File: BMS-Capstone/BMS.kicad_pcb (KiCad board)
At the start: 2 copper layers, 92.7 x 127 mm, 146 parts, among them IC1 BQ7694204PFBR, IC1 MP2643, IC2 MP2643, IC3 MP2643, IC4 MP2643, IC5 MP2643, IC6 MP2643, J1 Conn_01x02_Socket, J2 Conn_01x02_Socket, J3 Conn_01x13_Socket, K1 J107F1CS203VDC.80, Q1 FODM121, Q10 FODM121, Q11 FODM121, Q12 FODM121, Q2 FODM121, Q3 FODM121, Q4 FODM121, Q5 FODM121, Q6 FODM121, Q7 FODM121, Q8 FODM121, Q9 FODM121, U1 Teensy4.0

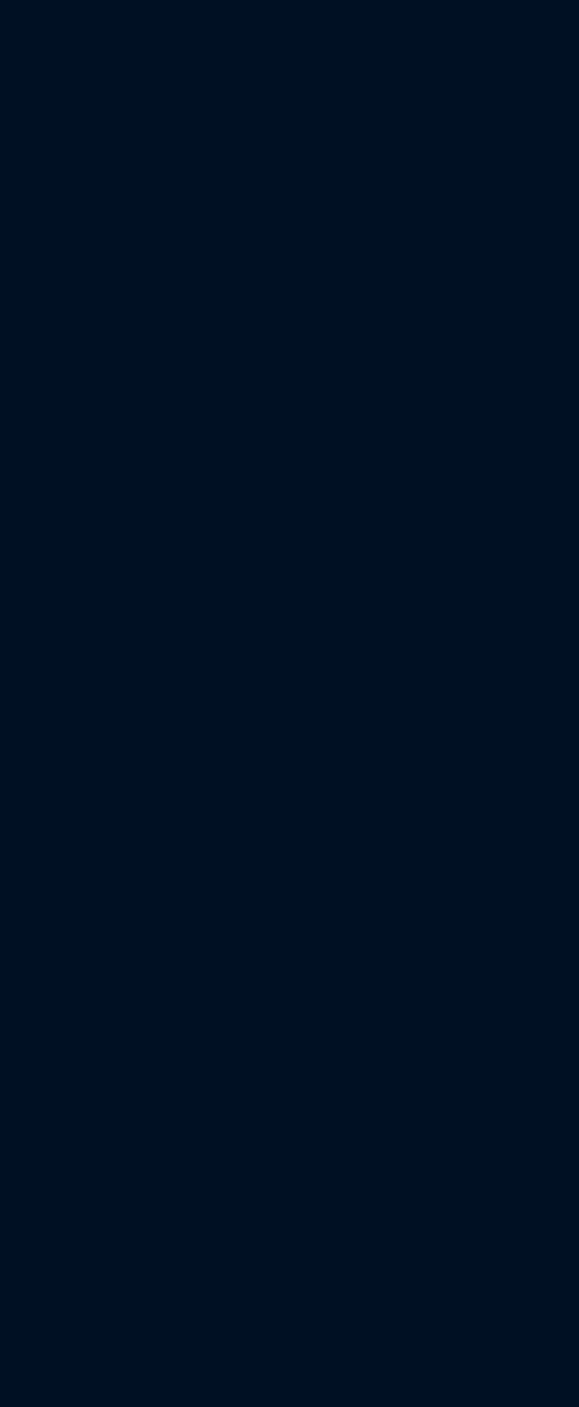
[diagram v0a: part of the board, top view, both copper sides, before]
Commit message: relinked footprints
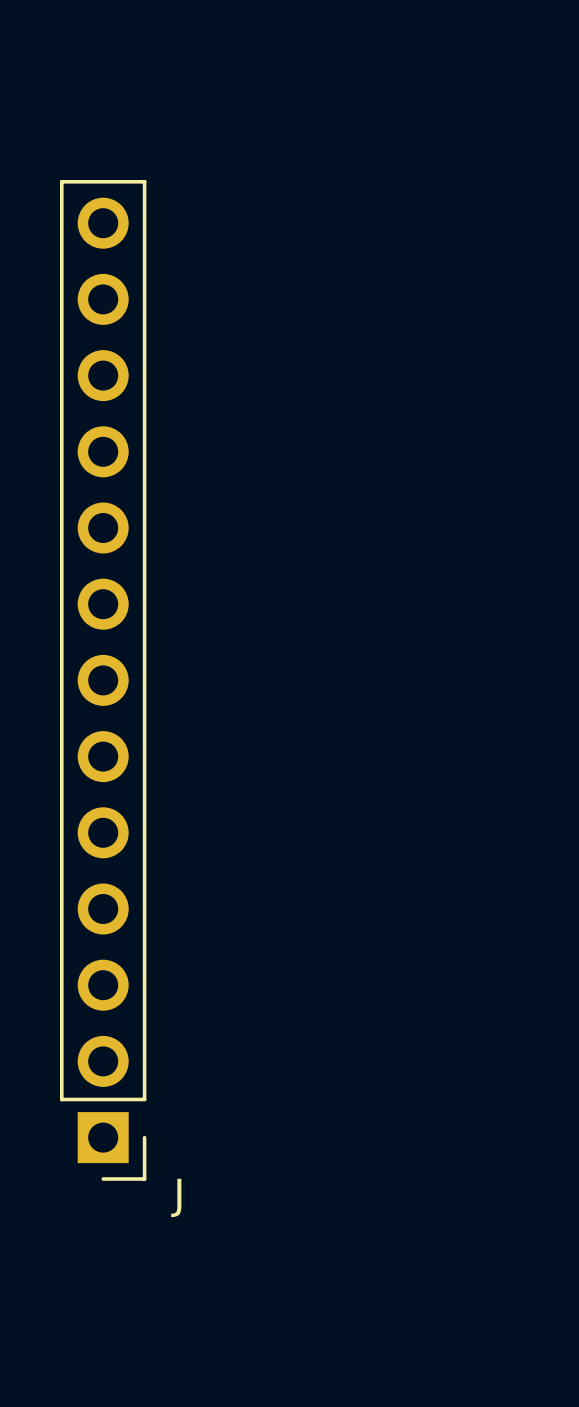
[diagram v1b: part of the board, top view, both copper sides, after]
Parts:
- added J: Conn_01x13_Socket, Connector_PinHeader_2.54mm:PinHeader_1x13_P2.54mm_Vertical, F.Cu at (27.3, 90.2)
